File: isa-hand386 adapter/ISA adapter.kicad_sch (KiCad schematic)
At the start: 16 parts, among them J1 Conn_02x30_Odd_Even, J2 Conn_02x30_Odd_Even, J3 Bus_ISA_8bit, J4 IRQDMA_JP, J5 Wavetable, J6 AudioJack3, U1 74HC14

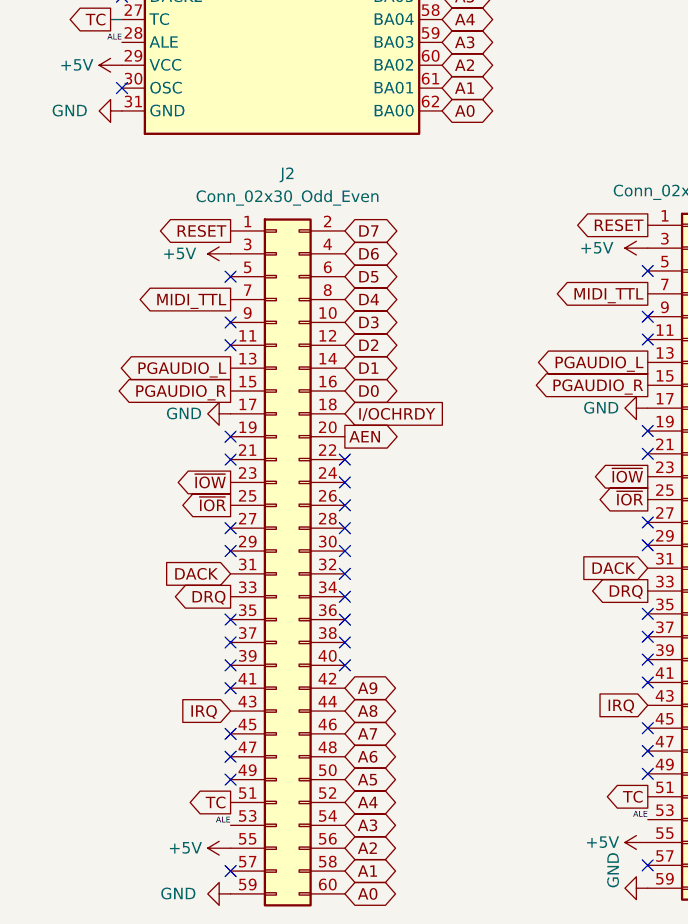
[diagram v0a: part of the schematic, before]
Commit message: Hand386 version and ISA adapter fabbed at JLC 8/25
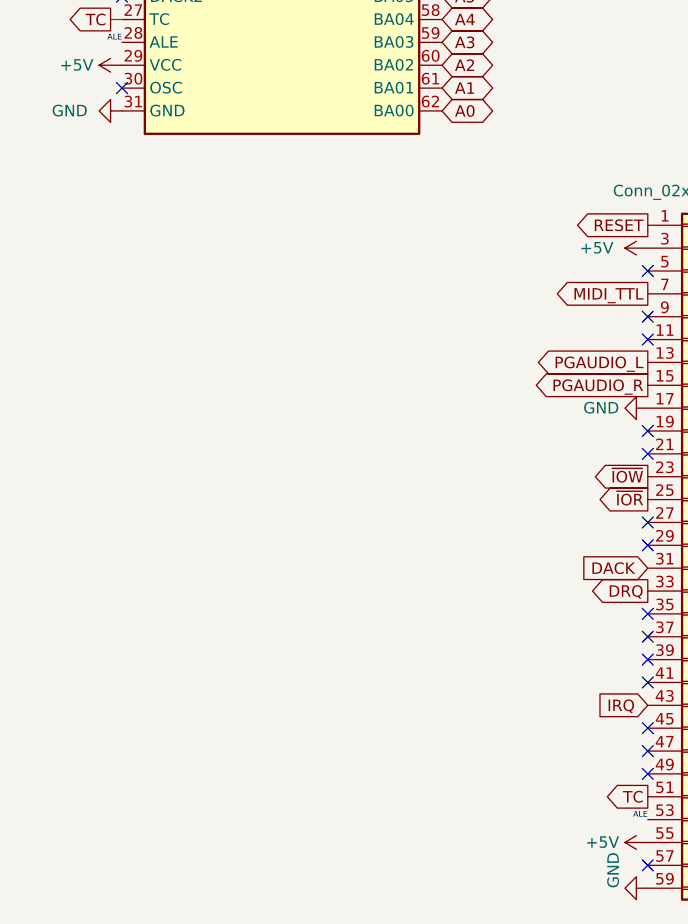
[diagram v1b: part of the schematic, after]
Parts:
- removed J2: Conn_02x30_Odd_Even, PiGUS library:Hand386_PicoGUS, symbol Connector_Generic:Conn_02x30_Odd_Even
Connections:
- no-connect marks 75 -> 50
